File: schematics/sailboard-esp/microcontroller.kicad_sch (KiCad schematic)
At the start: 2 parts

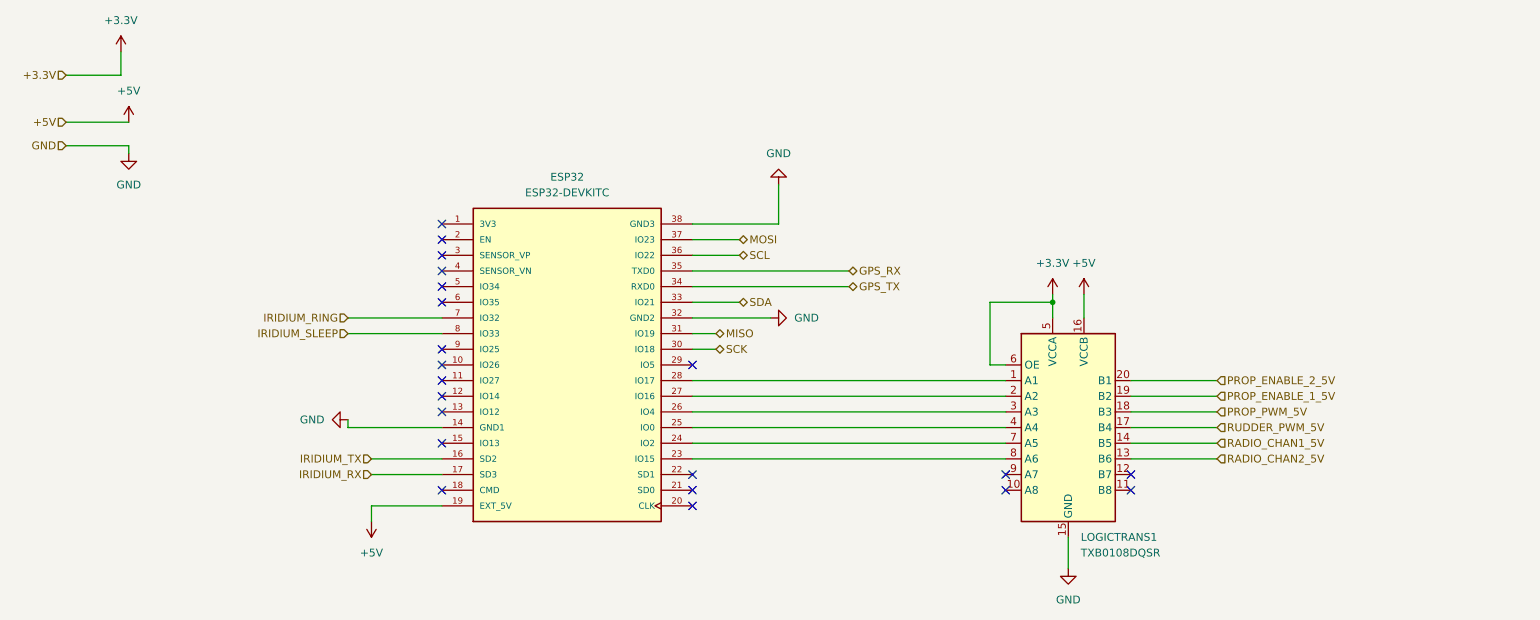
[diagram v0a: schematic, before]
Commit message: v1.1 of sailboard.
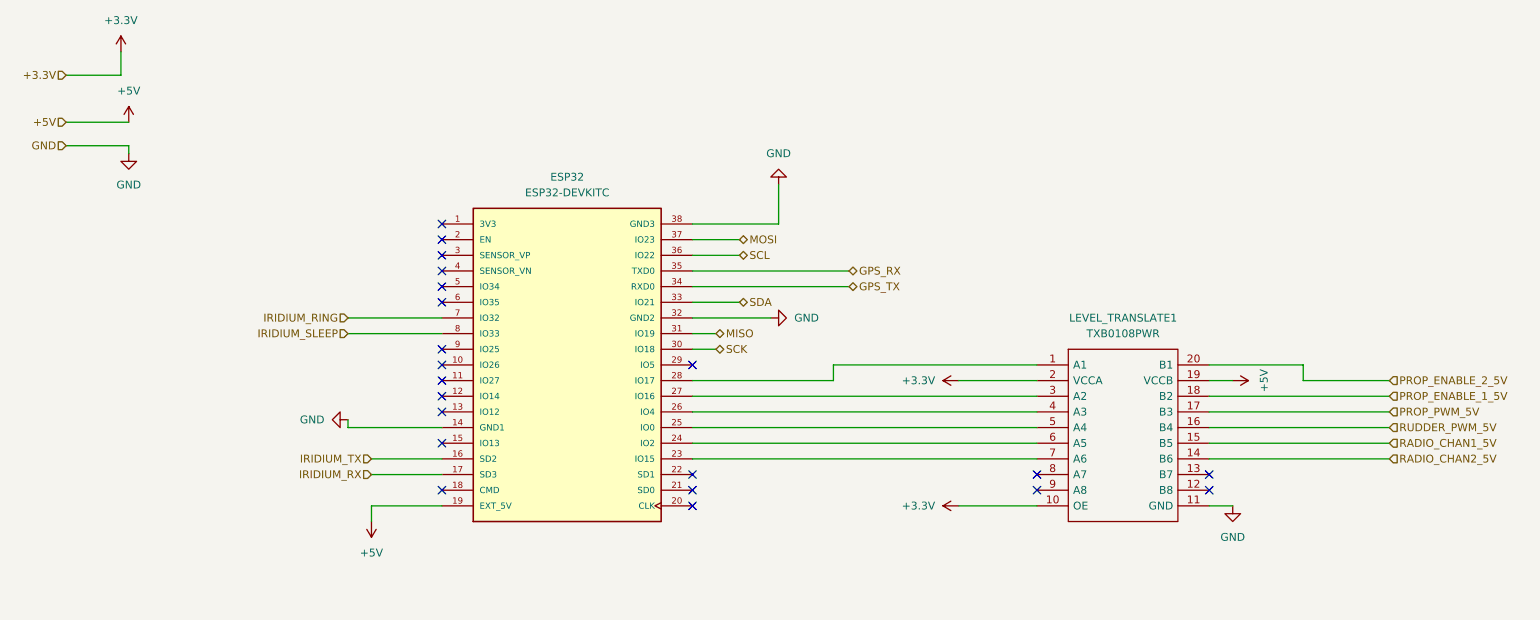
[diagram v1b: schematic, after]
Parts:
- removed LOGICTRANS1: TXB0108DQSR, Package_SON:USON-20_2x4mm_P0.4mm, symbol Logic_LevelTranslator:TXB0108DQSR
- added LEVEL_TRANSLATE1: TXB0108PWR, SOP65P640X120-20N, symbol TXB0108PWR:TXB0108PWR
- ESP32: footprint MODULE_ESP32-DEVKITC -> ESP32-DEVKITC:MODULE_ESP32-DEVKITC-RESIZED
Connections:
- net +3.3V: now also LEVEL_TRANSLATE1.10 (OE), LEVEL_TRANSLATE1.2 (VCCA)
- net +5V: now also LEVEL_TRANSLATE1.19 (VCCB)
- net GND: now also LEVEL_TRANSLATE1.11 (GND)
- net PROP_ENABLE_1_5V: now also LEVEL_TRANSLATE1.18 (B2)
- net PROP_ENABLE_2_5V: now also LEVEL_TRANSLATE1.20 (B1)
- net PROP_PWM_5V: now also LEVEL_TRANSLATE1.17 (B3)
- net RADIO_CHAN1_5V: now also LEVEL_TRANSLATE1.15 (B5)
- net RADIO_CHAN2_5V: now also LEVEL_TRANSLATE1.14 (B6)
- net RUDDER_PWM_5V: now also LEVEL_TRANSLATE1.16 (B4)
- net at ESP32.28 (IO17): now also LEVEL_TRANSLATE1.1 (A1)
- net at ESP32.27 (IO16): now also LEVEL_TRANSLATE1.3 (A2)
- net at ESP32.26 (IO4): now also LEVEL_TRANSLATE1.4 (A3)
- net at ESP32.25 (IO0): now also LEVEL_TRANSLATE1.5 (A4)
- net at ESP32.24 (IO2): now also LEVEL_TRANSLATE1.6 (A5)
- net at ESP32.23 (IO15): now also LEVEL_TRANSLATE1.7 (A6)
